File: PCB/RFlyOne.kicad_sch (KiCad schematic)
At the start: 74 parts, among them J1 UFL, Q1 AO3401A, U1 TQP3M9036, U10 ATGM332D-5N31, U2 TLV3201, U3 TA0970A, U4 TQP3M9036, U5 TA0970A, U6 AD8313ARMZ, U7 RP2040, U8 W25Q128, U9 12MHz

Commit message: checkpoint
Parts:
- added BT1: BAT, symbol Device:Battery_Cell
- added C30, C31, C40, C43: 1uF, Capacitor_SMD:C_0402_1005Metric, symbol Device:C_Small
- added C32: 22nF, Capacitor_SMD:C_0402_1005Metric, symbol Device:C_Small
- added C33, C35, C36, C39, C45, C46, C48, C49, C50: 10uF, Capacitor_SMD:C_0603_1608Metric, symbol Device:C_Small
- added C34: 22uF, Capacitor_SMD:C_0603_1608Metric, symbol Device:C_Small
- added C37, C38, C41, C42, C52, C54, C55, C56: 0.1uF, Capacitor_SMD:C_0402_1005Metric, symbol Device:C_Small
- added C44: 47nF, Capacitor_SMD:C_0402_1005Metric, symbol Device:C_Small
- added C47: 4.7uF, Capacitor_SMD:C_0402_1005Metric, symbol Device:C_Small
- added C51, C53: 22uF, Capacitor_SMD:C_0805_2012Metric, symbol Device:C_Small
- added Card1: TF-115-BCP9, easyeda2kicad:TF-SMD_TF-115-BCP9, symbol RFlyOne:TF-115-BCP9
- added D3: USBLC6-2SC6, easyeda2kicad:SOT-23-6_L2.9-W1.6-P0.95-LS2.8-BL, symbol RFlyOne:USBLC6-2SC6
- added D4: WHITE, symbol Device:LED_Small
- added JP1: ChargeDisable, symbol Jumper:SolderJumper_2_Open
- added L5, L6, L7: 1.5uH, Inductor_SMD:L_Changjiang_FTC201610S, symbol Device:L_Small
- added Q2: AO3401A, Package_TO_SOT_SMD:SOT-23, symbol Transistor_FET:AO3401A
- added R18, R19: 5.1k, Resistor_SMD:R_0402_1005Metric, symbol Device:R_Small
- added R20, R23, R24, R25, R28, R30, R31, R32, R34: 10k, Resistor_SMD:R_0402_1005Metric, symbol Device:R_Small
- added R21: 45.3k, Resistor_SMD:R_0402_1005Metric, symbol Device:R_Small
- added R22: 2.7k, Resistor_SMD:R_0402_1005Metric, symbol Device:R_Small
- added R26, R33: 160R, Resistor_SMD:R_0402_1005Metric, symbol Device:R_Small
- added R27: 330R, Resistor_SMD:R_0402_1005Metric, symbol Device:R_Small
- added R29: 73.2k, Resistor_SMD:R_0402_1005Metric, symbol Device:R_Small
- added SW1: TS24CA, easyeda2kicad:SW-SMD_2P-TS24CA, symbol RFlyOne:TS24CA
- added TP9: CH32_SWDIO, symbol Connector:TestPoint
- added U11: ESP32_S3_MINI, RF_Module:ESP32-S2-MINI-1U, symbol RF_Module:ESP32-S3-MINI-1U
- added U12: E80-900M2212S, easyeda2kicad:WIRELM-SMD_E80-900M2212S, symbol RFlyOne:E80-900M2212S_C55338904
- added U13: RT9193-33GB, easyeda2kicad:SOT-23-5_L3.0-W1.7-P0.95-LS2.8-BL, symbol RFlyOne:RT9193-33GB
- added U14: RT8097CHGE, easyeda2kicad:SOT-23-6_L2.9-W1.6-P0.95-LS2.8-BL, symbol RFlyOne:RT8097CHGE
- added U15: BMI270, easyeda2kicad:LGA-14_L3.0-W2.5-P0.50-BR, symbol RFlyOne:BMI270
- added U16: MMC5983MA, easyeda2kicad:LGA-16_L3.0-W3.0-P0.50-BL_SQ, symbol RFlyOne:MMC5983MA
- added U17: BQ25606RGER, easyeda2kicad:VQFN-24_L4.0-W4.0-P0.50-TL-EP2.8, symbol RFlyOne:BQ25606RGER
- added U18: TPS61023DRLR, easyeda2kicad:SOT-563_L1.6-W1.2-P0.50-LS1.6-BR, symbol RFlyOne:TPS61023DRLR
- added U19: CH32V003F4U6, easyeda2kicad:QFN-20_L3.0-W3.0-P0.40-TL-EP1.7, symbol RFlyOne:CH32V003F4U6
- added U20: TXU0202DTTR, easyeda2kicad:XSON-8_L2.0-W1.0-P0.50-BL, symbol RFlyOne:TXU0202DTTR
- added USB2: CONN_USB_C, easyeda2kicad:USB-C-SMD_TYPE-C-6PIN-2MD-073, symbol RFlyOne:TYPE-C16PIN2MD(073)
- Q1: now in the parts list
- TP1, TP2, TP3, TP4, TP5, TP6, TP8: now left out of the parts list
- TP7: value ESP_UART_TX -> ESP_UART_RX; now left out of the parts list
- USB1: value TYPE-C 16PIN 2MD(073) -> CONN_USB_C; footprint lcsc:USB-C-SMD_TYPE-C-6PIN-2MD-073 -> easyeda2kicad:USB-C-SMD_TYPE-C-6PIN-2MD-073
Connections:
- net +3V3: now also C31.1, U13.5 (VOUT); no longer C18.1, C19.1, C20.1, C21.1, C22.1, C23.1, C24.1, R12.2, R14.2, U7.1 (IOVDD), U7.10 (IOVDD), U7.22 (IOVDD), U7.33 (IOVDD), U7.42 (IOVDD), U7.43 (ADC_AVDD), U7.44 (VREG_IN), U7.48 (USB_VDD), U7.49 (IOVDD), U8.8 (VCC)
- net +5V: now also C30.1, C33.1, C51.1, C52.1, C53.1, R29.2, U13.1 (VIN), U13.3 (EN), U14.1 (EN), U14.4 (VIN), U18.6 (VOUT); no longer D2.5, USB1.11 (VBUS), USB1.2 (VBUS)
- net GND: now also BT1.2 (-), C30.2, C31.2, C32.2, C33.2, C34.2, C35.2, C36.2, C37.2, C38.2, C39.2, C40.2, C41.2, C42.2, C43.2, C45.2, C46.2, C47.2, C48.2, C49.2, C50.2, C51.2, C52.2, C53.2, C54.2, C55.1, C56.2, D3.2, R18.2, R19.2, R20.2, R24.2, R25.1, R26.1, R27.1, R28.1, R34.1, U11.1 (GND), U11.2 (GND), U11.42 (GND), U11.43 (GND), U11.46 (GND), U11.47 (GND), U11.48 (GND), U11.49 (GND), U11.50 (GND), U11.51 (GND), U11.52 (GND), U11.53 (GND), U11.54 (GND), U11.55 (GND), U11.56 (GND), U11.57 (GND), U11.58 (GND), U11.59 (GND), U11.60 (GND), U11.61 (GND), U11.62 (GND), U11.63 (GND), U11.64 (GND), U11.65 (GND), U13.2 (GND), U14.2 (GND), U15.1 (SDO), U15.6 (GNDIO), U15.7 (GND), U16.11 (GND), U16.9 (GND), U17.17 (GND), U17.18 (GND), U17.25 (EP), U17.6 (OTG), U18.4 (GND), U19.21 (VSS), U19.4 (VSS), U20.2 (GND), USB2.1 (GND), USB2.12 (GND), USB2.13 (SHELL), USB2.14 (SHELL)
- net USB_DM renamed CONN_RP_USB_DM
- net USB_DP renamed CONN_RP_USB_DP
- new net: Q2.1 (G), R32.1, R33.1
- new net: R33.2, U19.8 (PC1)
- new net: R19.1, USB2.10 (CC2)
- new net: C44.2, L6.1, U17.19 (SW), U17.20 (SW)
- new net: R27.2, U17.10 (ICHG)
- new net: R26.2, U17.8 (ILIM)
- new net: R34.2, TP9.1, U19.15 (PD1)
- new net: R20.1, R21.2, U14.6 (FB)
- new net: C32.1, U13.4 (BP)
- new net: L5.1, U14.3 (LX)
- new net: R18.1, USB2.4 (CC1)
- new net: BT1.1 (+), C46.1, U17.13 (BAT), U17.14 (BAT)
- new net: C39.1, U16.10 (CAP)
- new net: C44.1, U17.21 (BTST)
- new net: L7.2, U18.5 (SW)
- new net +5VU: C43.1, D2.5, D3.5, U17.1 (VAC), U17.24 (VBUS), USB1.11 (VBUS), USB1.2 (VBUS), USB2.11 (VBUS), USB2.2 (VBUS)
- new net +BATT: C50.1, L7.1, Q2.3 (D), U18.2 (EN), U18.3 (VIN)
- new net +D3V3: C18.1, C19.1, C20.1, C21.1, C22.1, C23.1, C24.1, C34.1, C35.1, C36.1, C37.1, C38.1, C40.1, C41.1, C42.1, C56.1, L5.2, R12.2, R14.2, R21.1, U11.3 (3V3), U15.12 (CSB), U15.5 (VDDIO), U15.8 (VDD), U16.13 (VDDIO), U16.2 (VDD), U16.4 (SPI_CS), U20.6 (OE), U20.7 (VCCB), U7.1 (IOVDD), U7.10 (IOVDD), U7.22 (IOVDD), U7.33 (IOVDD), U7.42 (IOVDD), U7.43 (ADC_AVDD), U7.44 (VREG_IN), U7.48 (USB_VDD), U7.49 (IOVDD), U8.8 (VCC)
- new net BOOST_FB: R28.2, R29.1, U18.1 (FB)
- new net CE: JP1.1 (A), R25.2, U17.9 (~{CE})
- new net CH32_RX: U20.4 (A2Y)
- new net CH32_TX: U20.5 (A1)
- new net CHARGE: R30.1, U17.5 (STAT), U19.10 (PC3)
- new net CONN_ESP_USB_DM: D3.3, USB2.5 (DN2), USB2.7 (DN1)
- new net CONN_ESP_USB_DP: D3.1, USB2.6 (DP1), USB2.8 (DP2)
- new net ESP32_RX: U20.8 (B1Y)
- new net ESP32_TX: U20.1 (B2)
- new net ESP_USB_DM: D3.4, U11.23 (USB_D-)
- new net ESP_USB_DP: D3.6, U11.24 (USB_D+)
- new net PG: R31.1, U17.7 (~{PG}), U19.9 (PC2)
- new net PMID: C48.1, U17.23 (PMID)
- new net REGN: C47.1, JP1.2 (B), R23.1, U17.22 (REGN)
- new net SCL: U15.13 (SCX), U16.1 (SCL/SPI_SCK)
- new net SDA: U15.14 (SDX), U16.16 (SDA/SPI_SDI)
- new net SYSTEM: C45.1, C49.1, C54.1, C55.2, L6.2, Q2.2 (S), R30.2, R31.2, R32.2, U17.15 (SYS), U17.16 (SYS), U19.6 (VDD), U20.3 (VCCA)
- new net TS: R23.2, R24.1, U17.11 (TS)
- no-connect marks 24 -> 64
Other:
- note added: "1090MHz RF Frontend"
- note added: "5V Boost Converter"
- note added: "Charge Controller"
- note added: "Clean 3.3V"
- note added: "Digital 3.3V"
- note added: "IMU"
- note added: "Logic Level Translator"
- note added: "Magnetometer"
- note added: "USB Connector"
- moved on the sheet: C1, C10, C11, C12, C13, C14, C15, C16, C17, C18, C19, C2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

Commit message: checkpoint
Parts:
- added C57, C60: 0.1uF, Capacitor_SMD:C_0402_1005Metric, symbol Device:C_Small
- added C58, C59: 1uF, Capacitor_SMD:C_0402_1005Metric, symbol Device:C_Small
- added J2: UFL, easyeda2kicad:UFL, symbol Connector:Conn_Coaxial_Small
- added L8: 77nH, Inductor_SMD:L_0402_1005Metric, symbol Device:L_Small
- added R35, R36, R37, R38, R39, R40: 10k, Resistor_SMD:R_0402_1005Metric, symbol Device:R_Small
- added U21: TPS7A0230-3V0, easyeda2kicad:SOT-23-5_L2.9-W1.6-P0.95-LS2.8-BR, symbol RFlyOne:TPS7A0230PDBVR
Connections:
- net +D3V3: now also Card1.4 (VDD), U10.23 (VCC), C57.2, C60.1, R35.2, R36.2, R37.2, R38.2, R39.2, R40.2
- net GND: now also Card1.10 (GND), Card1.11 (GND), Card1.12 (GND), Card1.13 (GND), Card1.6 (VSS), U10.10 (GND), U10.12 (GND), U10.13 (GND), U10.24 (GND), C57.1, C58.2, C59.2, C60.2, J2.2 (Ext), U21.2 (GND)
- net SYSTEM: now also C58.1, U21.1 (IN), U21.3 (EN)
- net at U10.11 (RF_IN): now also J2.1 (In), L8.1
- net GNSS_TX: now reaches U10.20 (TXD1)
- net GNSS_RX: now reaches U10.21 (RXD1)
- net +3V0: now reaches U10.22 (VBAT)
- net +3V0: now also C59.1, U21.5 (OUT)
- net PPS: now reaches U10.3 (1PPS)
- net at U10.9 (VCC_RF): now also L8.2
- net SDIO_DAT2: now reaches Card1.1 (DATA2)
- net SDIO_DAT2: now also R37.1
- net SDIO_DAT3: now reaches Card1.2 (CD/DATA3)
- net SDIO_DAT3: now also R38.1
- net SDIO_CMD: now reaches Card1.3 (CMD)
- net SDIO_CMD: now also R39.1
- net SDIO_CLK: now reaches Card1.5 (CLK)
- net SDIO_DAT0: now reaches Card1.7 (DAT0)
- net SDIO_DAT0: now also R35.1
- net SDIO_DAT1: now reaches Card1.8 (DAT1)
- net SDIO_DAT1: now also R36.1
- net SDIO_CD: now reaches Card1.9 (CD)
- net SDIO_CD: now also R40.1
- no-connect marks 64 -> 68
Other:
- note added: "GNSS Module"
- note added: "RP2040 16MB Flash"
- note added: "RTC LDO"
- note added: "SD Card Slot"
- moved on the sheet: C18, C19, C20, C21, C22, C23, C24, C25, C26, C27, C28, C29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

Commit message: checkpoint
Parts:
- added C61: 10uF, Capacitor_SMD:C_0603_1608Metric, symbol Device:C_Small
- added C62, C63: 0.1uF, Capacitor_SMD:C_0402_1005Metric, symbol Device:C_Small
- added R41, R44, R45: 10k, Resistor_SMD:R_0402_1005Metric, symbol Device:R_Small
- added R42: 2.7k, Resistor_SMD:R_0402_1005Metric, symbol Device:R_Small
- added R43: 7.5k, Resistor_SMD:R_0402_1005Metric, symbol Device:R_Small
- added SW2, SW4, SW5: TS24CA, easyeda2kicad:SW-SMD_2P-TS24CA, symbol RFlyOne:TS24CA
- added TP10: ESP_RST, symbol Connector:TestPoint
- added U22: 240x240_1.3in_TFT, easyeda2kicad:1.3TFT, symbol RFlyOne:TFT_1.3
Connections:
- net +BATT: now also R43.2
- net +D3V3: now also R22.2, U12.25 (VCC), C61.1, C62.1, R41.1, R42.2, R45.2, U22.2 (VCC)
- net BIAS_TEE_EN: no longer U7.29 (GPIO18)
- net CHARGE: now also R31.1; no longer R30.1, U19.10 (PC3)
- net GND: now also U12.1 (GND), U12.11 (GND), U12.13 (GND), U12.14 (GND), U12.16 (GND), U12.19 (GND), U12.26 (GND), U12.8 (GND), C61.2, C62.2, C63.2, R44.1, SW2.2, SW2.3, SW2.4, SW4.2, SW4.3, SW4.4, SW5.2, SW5.3, SW5.4, U22.1 (GND)
- net PG: now also R30.1; no longer R31.1, U19.9 (PC2)
- net PULSE: no longer U7.30 (GPIO19)
- net SCL: now also R42.1
- net SDA: now also R22.1
- net at U7.36 (GPIO24): no longer TP1.1
- net at U7.6 (GPIO4): no longer TP5.1
- net at U7.7 (GPIO5): no longer TP6.1
- net at U12.21 (LR_NRESET): now also R41.2
- net LORA_MISO: now reaches U12.3 (MISO)
- net LORA_MOSI: now reaches U12.4 (MOSI)
- net LORA_SCK: now reaches U12.5 (SCK)
- net LORA_CE: now reaches U12.6 (NSS)
- net LORA_BUSY: now reaches U12.7 (BUSY)
- net at U11.45 (EN): now also R45.1, TP10.1
- net ESP32_RX renamed BTMGR_ESP32_RX
- net ESP32_TX renamed BTMGR_ESP32_TX
- net ESP_UART_RX: no longer names the net of U7.28 (GPIO17)
- net ESP_UART_RX: no longer TP7.1
- net ESP_UART_TX: no longer names the net of U7.27 (GPIO16)
- net ESP_UART_TX: no longer TP8.1
- new net BATT_ADC: C63.1, R43.1, R44.2
- new net LCD_BRIGHT: U22.7 (BLK)
- new net LCD_CMD: U22.6 (DC)
- new net LCD_MOSI: U22.4 (SDA)
- new net LCD_RST: U22.5 (RES)
- new net LCD_SDK: U22.3 (SCL)
- new net LEFT_BTN: SW2.1
- new net OK_BTN: SW4.1
- new net RIGHT_BTN: SW5.1
- no-connect marks 68 -> 79
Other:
- note added: "LCD Display"
- note added: "LEFT"
- note added: "LoRa Module"
- note added: "OK"
- note added: "RIGHT"
- note added: "Temporarily Unconnected"
- moved on the sheet: C18, C19, C20, C21, C22, C23, C24, C25, C26, C27, C28, C29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

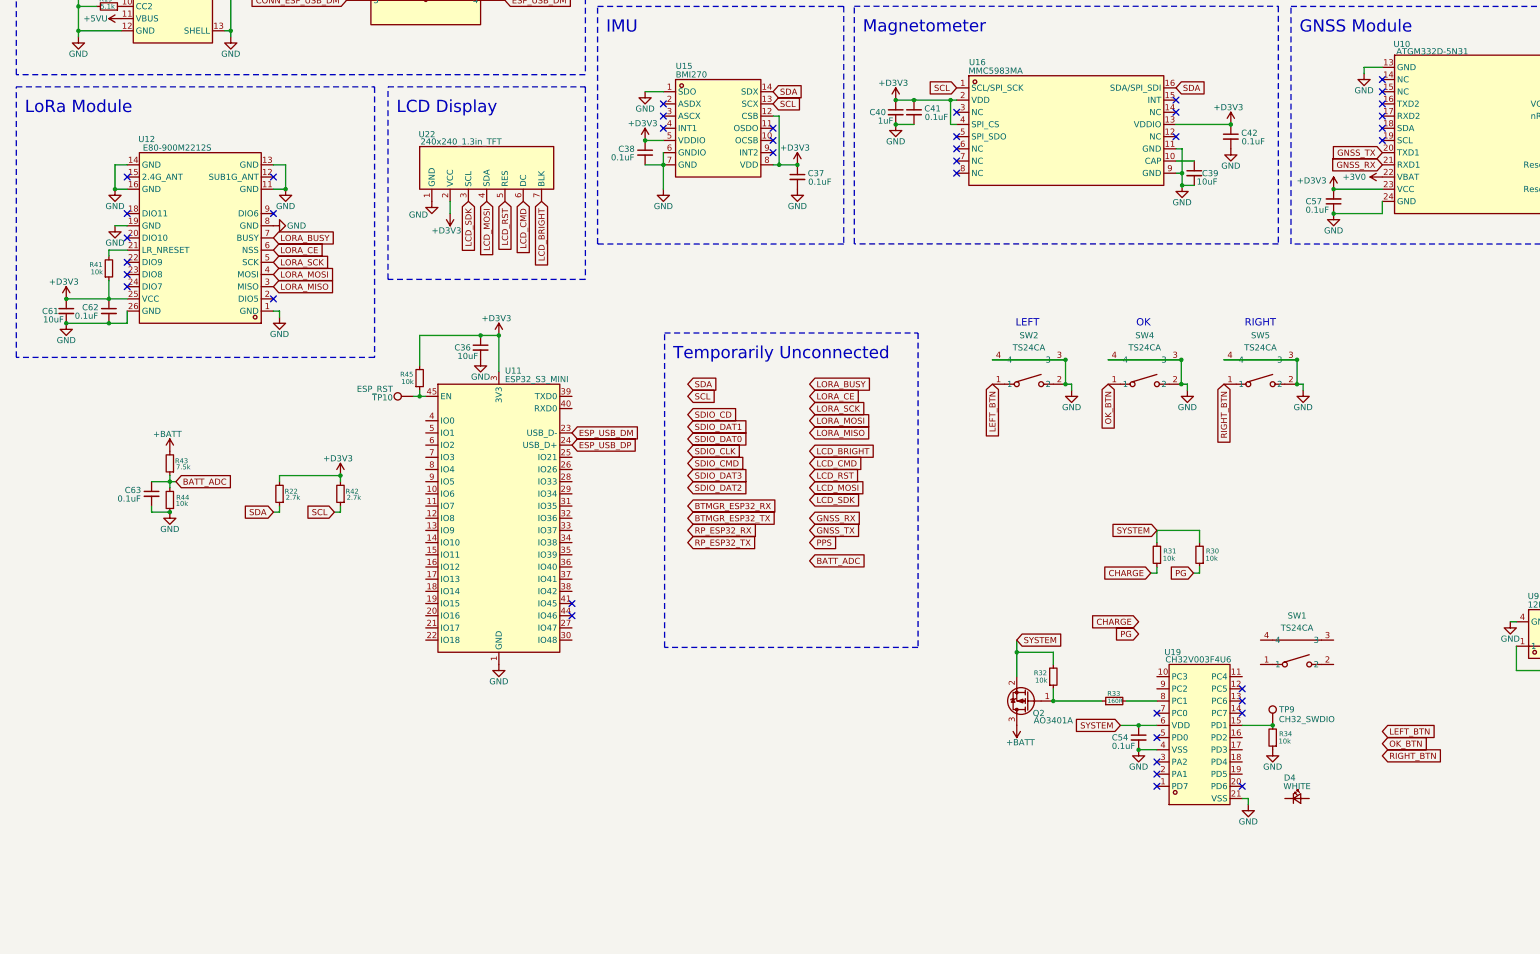
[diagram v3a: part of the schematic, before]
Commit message: checkpoint
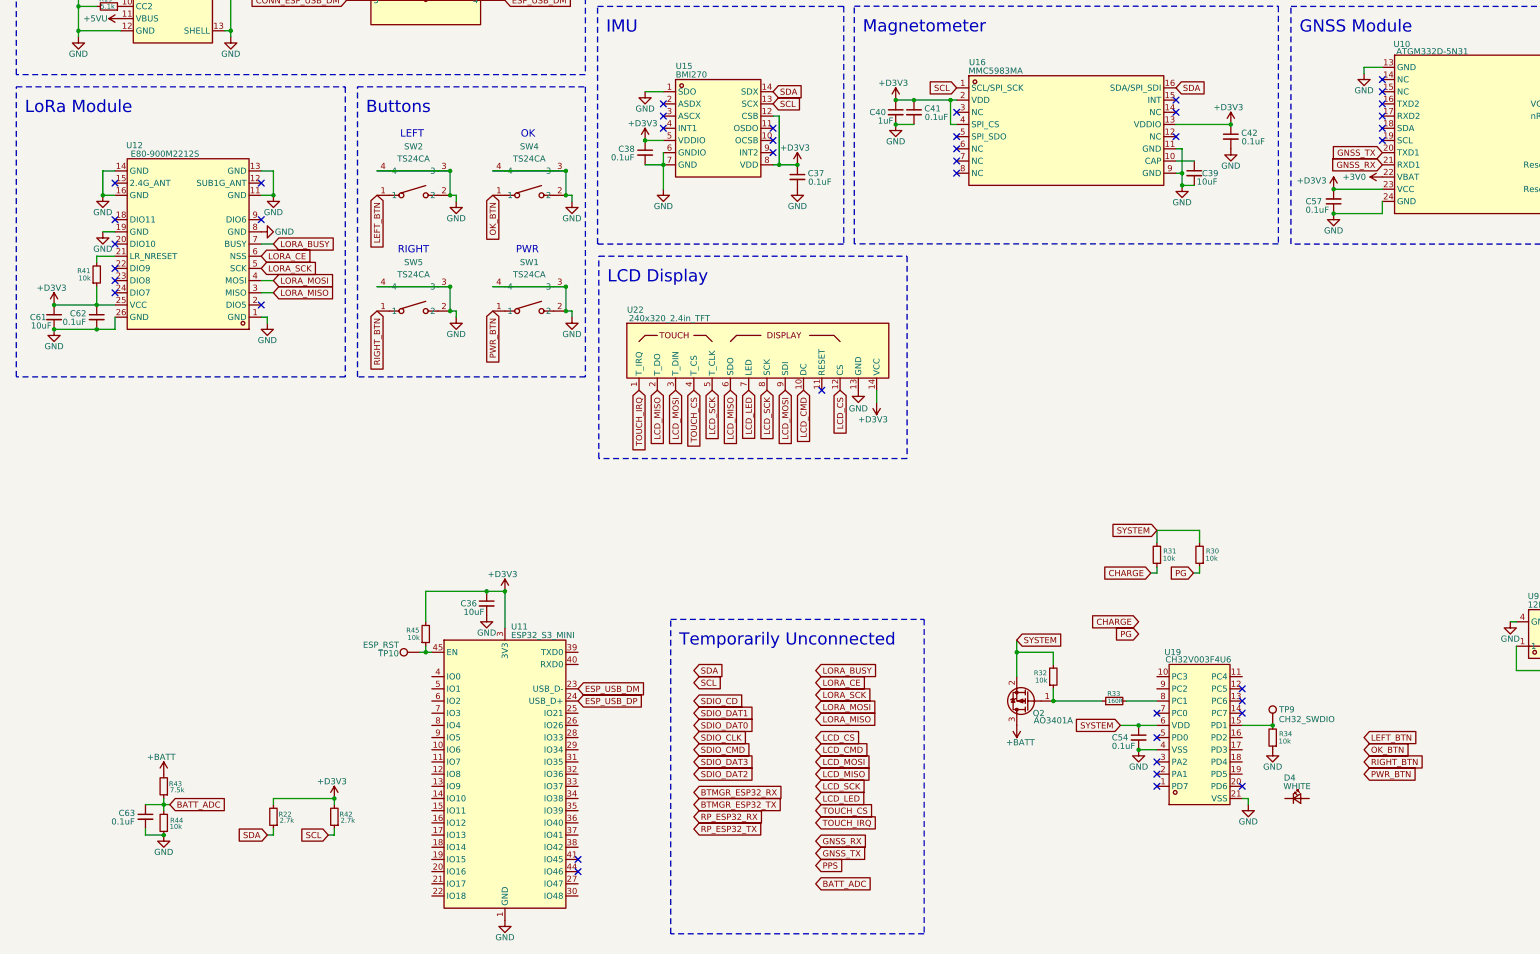
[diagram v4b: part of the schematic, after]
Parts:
- removed U22: 240x240_1.3in_TFT, easyeda2kicad:1.3TFT, symbol RFlyOne:TFT_1.3
- added U22: 240x320_2.4in_TFT, easyeda2kicad:2.4TFT, symbol RFlyOne:TFT_2.4
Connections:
- net +D3V3: now also U22.14 (VCC)
- net GND: now also SW1.2, SW1.3, SW1.4, U22.13 (GND)
- net LCD_CMD: now also U22.10 (DC)
- net LCD_MOSI: now also U22.3 (T_DIN), U22.9 (SDI)
- net PWR_BTN: now reaches SW1.1
- new net LCD_CS: U22.12 (CS)
- new net LCD_LED: U22.7 (LED)
- new net LCD_MISO: U22.2 (T_DO), U22.6 (SDO)
- new net LCD_SCK: U22.5 (T_CLK), U22.8 (SCK)
- new net TOUCH_CS: U22.4 (T_CS)
- new net TOUCH_IRQ: U22.1 (T_IRQ)
- no-connect marks 79 -> 80
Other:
- note added: "Buttons"
- note added: "PWR"
- moved on the sheet: C36, C61, C62, C63, R22, R41, R42, R43, R44, R45, SW2, SW4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
